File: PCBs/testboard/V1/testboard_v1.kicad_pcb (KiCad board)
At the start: 2 copper layers, 39 parts, among them J1 FLEX pin1, J10 Conn_01x01, J11 Conn_01x01, J12 Conn_01x01, J13 Conn_01x02_Socket, J2 FLEX pin2, J3 FSR pin2, J4 FSR pin1, J5 Conn_01x02_Socket, J9 Conn_01x01, Q1 BSS138, Q2 BSS138, U1 ICM-20948, U2 STM32F405RGTx, U3 TLV70018_SOT23-5

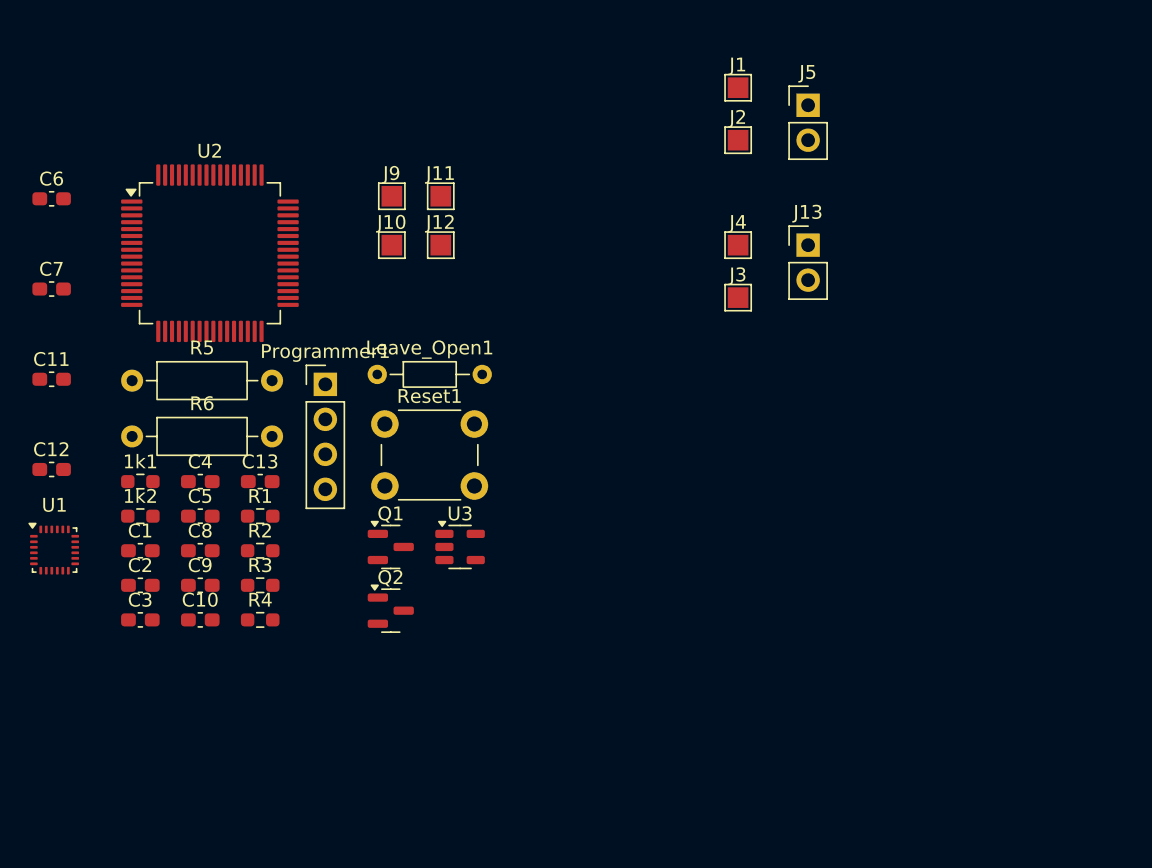
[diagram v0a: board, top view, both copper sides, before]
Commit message: V1 layout done (its kinda crappy tho)
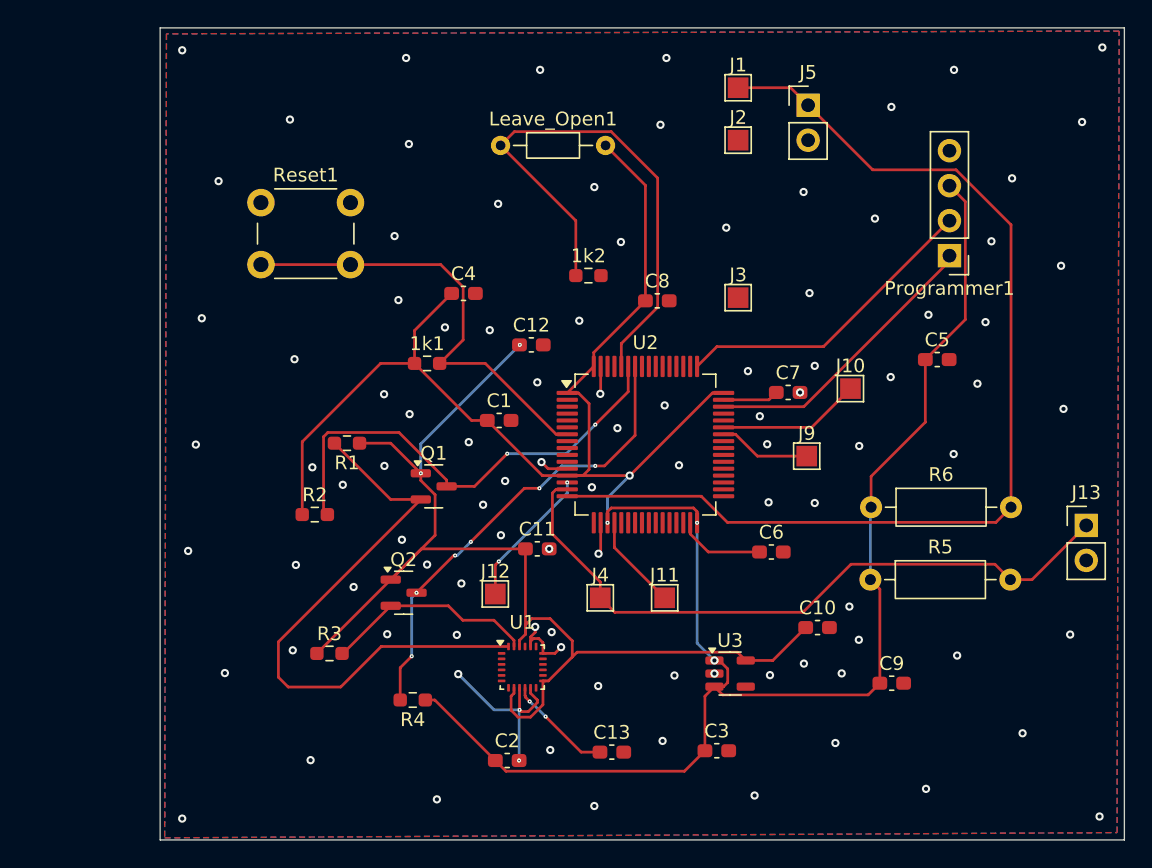
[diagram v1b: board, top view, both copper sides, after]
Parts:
- moved C6 58.2 mm to (177.7, 106.1)
- moved R5 55.5 mm to (184.9, 108.1)
- moved C5 54.7 mm to (189.7, 92.1)
- moved C7 54.0 mm to (178.9, 94.5)
- moved R6 53.9 mm to (184.9, 102.8)
- moved C9 50.7 mm to (186.4, 115.6)
- moved Programmer1 46.3 mm to (190.6, 84.6), turned to 180 degrees
- moved C10 44.8 mm to (181.0, 111.6)
- moved C3 42.9 mm to (173.7, 120.5)
- moved C8 37.8 mm to (169.4, 87.9)
- moved C11 37.3 mm to (160.7, 105.9)
- moved 1k2 36.9 mm to (164.4, 86.0)
- moved C12 36.0 mm to (160.2, 91.1)
- moved J9 35.5 mm to (180.2, 99.1)
- moved U1 35.0 mm to (159.6, 114.5)
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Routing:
- net VCC: track 0.00 -> 186.8 mm, vias 0 -> 4
- net /VLDO_OUT: track 0.00 -> 86.3 mm, vias 0 -> 2
- net /ADC_FLEX1: track 0.00 -> 77.9 mm
- net /ADC_FSR1: track 0.00 -> 49.5 mm
- net /SDA_1.8V: track 0.00 -> 43.4 mm
- net Net-(U2-BOOT0): track 0.00 -> 39.7 mm
- net /SDA: track 0.00 -> 34.6 mm, vias 0 -> 2
- net /SCL: track 0.00 -> 33.9 mm, vias 0 -> 6
- net Net-(U2-NRST): track 0.00 -> 33.0 mm
- net GND: track 0.00 -> 25.4 mm, vias 0 -> 99
- net /SWCLK: track 0.00 -> 22.7 mm
- net /SWDIO: track 0.00 -> 21.2 mm
- net /SCL_1.8V: track 0.00 -> 15.4 mm
- net /DEBUG_2: track 0.00 -> 10.4 mm
- net /DEBUG_4: track 0.00 -> 10.3 mm, vias 0 -> 2
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- added copper zone on B.Cu, net GND
- added copper zone on F.Cu, net GND
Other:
- board outline added: 70 x 59 mm
